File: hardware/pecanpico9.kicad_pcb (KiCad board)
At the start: 4 copper layers, 29.8 x 33.7 mm, 111 parts, among them IC1 SPV1040T, IC2 TPS62260DRVR, IC3 ADP322ACPZ-115-R7, IC4 Si4063-B1B-FM, IC5 STM32F413xG, IC6 EVA-7M, IC7 PAC1720-1-AIA-TR, IC8 LDLN015PU33R, IC9 BME280, P1 CONN_01X25, P2 CONN_01X10, P3 ZX62-B-5PA(33), P4 IPX 2mm, P5 CONN_01X02, P6 IPX 2mm, Q1 FDN306P, X1 KT2016K26000BCW18ZAS

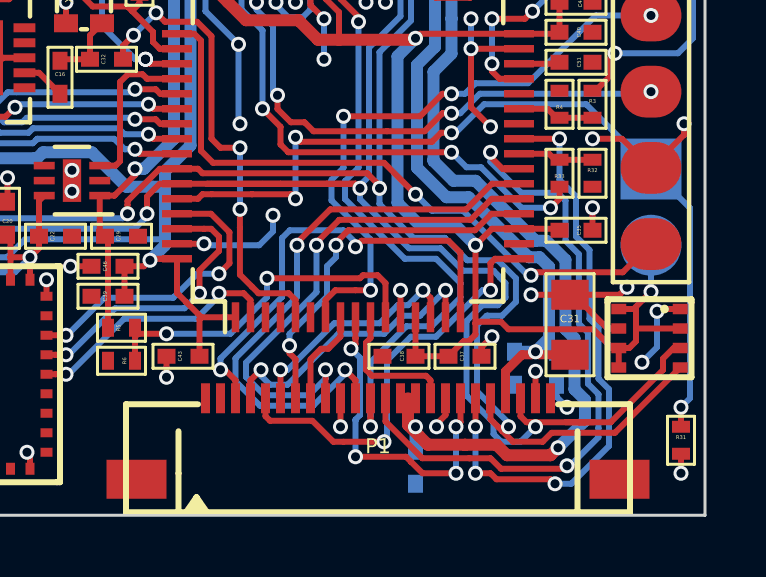
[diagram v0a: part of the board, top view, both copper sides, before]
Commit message: Wiggled parts around
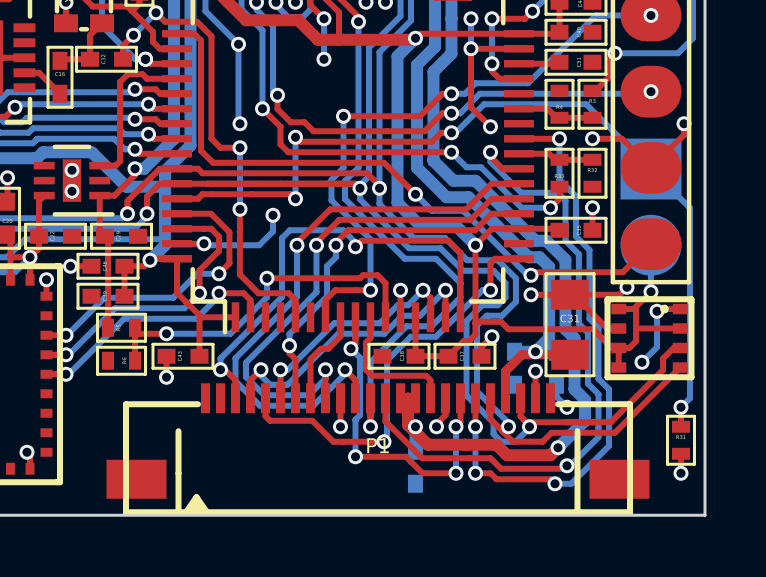
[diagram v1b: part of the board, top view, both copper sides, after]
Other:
- net class Default: clearance 0.15 -> 0.149
- rule trace_clearance: 0.15 -> 0.149
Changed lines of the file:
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@@
     (thickness 1)
     (drawings 30)
-    (tracks 1487)
+    (tracks 1489)
     (zones 0)
     (modules 111)
@@
   (setup
     (last_trace_width 0.2)
-    (trace_clearance 0.15)
+    (trace_clearance 0.149)
     (zone_clearance 0.15)
     (zone_45_only no)
@@
   (net 78 /CAM_PCLK)
   (net_class Default "This is the default net class."
-    (clearance 0.15)
+    (clearance 0.149)
     (trace_width 0.2)
     (via_dia 0.5)
@@
   (via (at 58.35 110.9) (size 0.5) (drill 0.3) (layers F.Cu B.Cu) (net 22))
   (via (at 53.9 111) (size 0.5) (drill 0.3) (layers F.Cu B.Cu) (net 22))
+  (segment (start 71.05 121.65) (end 71.05 121.690002) (width 0.2) (layer B.Cu) (net 23))
+  (segment (start 70.110479 122.149001) (end 69.850999 121.889521) (width 0.2) (layer B.Cu) (net 23))
+  (segment (start 70.249001 117.339521) (end 70.249001 116.860479) (width 0.2) (layer B.Cu) (net 23))
+  (segment (start 71.05 121.690002) (end 70.591001 122.149001) (width 0.2) (layer B.Cu) (net 23))
+  (segment (start 70.591001 122.149001) (end 70.110479 122.149001) (width 0.2) (layer B.Cu) (net 23))
+  (segment (start 69.850999 121.889521) (end 69.850999 121.512477) (width 0.2) (layer B.Cu) (net 23))
+  (segment (start 69.850999 121.512477) (end 68.95199 120.613468) (width 0.2) (layer B.Cu) (net 23))
+  (segment (start 70.249001 116.860479) (end 70.051374 116.662852) (width 0.2) (layer B.Cu) (net 23))
+  (segment (start 68.95199 118.12368) (end 69.476669 117.599001) (width 0.2) (layer B.Cu) (net 23))
+  (segment (start 68.95199 120.613468) (end 68.95199 118.12368) (width 0.2) (layer B.Cu) (net 23))
+  (segment (start 69.476669 117.599001) (end 69.989521 117.599001) (width 0.2) (layer B.Cu) (net 23))
+  (segment (start 69.849384 116.44801) (end 68.830106 116.44801) (width 0.2) (layer B.Cu) (net 23))
+  (segment (start 69.989521 117.599001) (end 70.249001 117.339521) (width 0.2) (layer B.Cu) (net 23))
+  (segment (start 70.051374 116.662852) (end 70.051374 116.65) (width 0.2) (layer B.Cu) (net 23))
+  (segment (start 70.051374 116.65) (end 69.849384 116.44801) (width 0.2) (layer B.Cu) (net 23))
+  (segment (start 68.830106 116.44801) (end 68.083095 115.700999) (width 0.2) (layer B.Cu) (net 23))
+  (segment (start 68.083095 115.700999) (end 67.035907 115.700999) (width 0.2) (layer B.Cu) (net 23))
+  (segment (start 67.035907 115.700999) (end 65.4 114.065092) (width 0.2) (layer B.Cu) (net 23))
+  (segment (start 65.4 114.065092) (end 65.4 113.7) (width 0.2) (layer B.Cu) (net 23))
+  (segment (start 70.951798 121.5) (end 70.851798 121.4) (width 0.2) (layer F.Cu) (net 23))
+  (segment (start 70.851798 121.4) (end 70.75 121.298202) (width 0.2) (layer F.Cu) (net 23))
+  (segment (start 71.05 121.65) (end 71.05 121.598202) (width 0.2) (layer F.Cu) (net 23))
+  (segment (start 71.05 121.598202) (end 70.851798 121.4) (width 0.2) (layer F.Cu) (net 23))
   (segment (start 65.4 113.7) (end 65.4 113.6) (width 0.2) (layer B.Cu) (net 23))
   (segment (start 65.7 109.017838) (end 65.94999 108.767848) (width 0.2) (layer B.Cu) (net 23))
@@
   (segment (start 60.3 113.55) (end 64.3 113.55) (width 0.2) (layer F.Cu) (net 23))
   (segment (start 64.3 113.55) (end 64.30099 113.54901) (width 0.2) (layer F.Cu) (net 23))
-  (segment (start 70.051374 116.662852) (end 70.249001 116.860479) (width 0.2) (layer B.Cu) (net 23))
-  (segment (start 65.4 113.7) (end 65.4 114.065092) (width 0.2) (layer B.Cu) (net 23))
-  (segment (start 69.989521 117.599001) (end 69.476669 117.599001) (width 0.2) (layer B.Cu) (net 23))
-  (segment (start 67.035907 115.700999) (end 68.083095 115.700999) (width 0.2) (layer B.Cu) (net 23))
-  (segment (start 69.849384 116.44801) (end 70.051374 116.65) (width 0.2) (layer B.Cu) (net 23))
-  (segment (start 65.4 114.065092) (end 67.035907 115.700999) (width 0.2) (layer B.Cu) (net 23))
-  (segment (start 68.083095 115.700999) (end 68.830106 116.44801) (width 0.2) (layer B.Cu) (net 23))
-  (segment (start 70.051374 116.65) (end 70.051374 116.662852) (width 0.2) (layer B.Cu) (net 23))
-  (segment (start 68.830106 116.44801) (end 69.849384 116.44801) (width 0.2) (layer B.Cu) (net 23))
-  (segment (start 69.476669 117.599001) (end 68.95199 118.12368) (width 0.2) (layer B.Cu) (net 23))
-  (segment (start 70.249001 116.860479) (end 70.249001 117.339521) (width 0.2) (layer B.Cu) (net 23))
-  (segment (start 70.249001 117.339521) (end 69.989521 117.599001) (width 0.2) (layer B.Cu) (net 23))
-  (segment (start 70.750999 122.149001) (end 71.25 121.65) (width 0.2) (layer B.Cu) (net 23))
-  (segment (start 68.95199 118.12368) (end 68.95199 120.613468) (width 0.2) (layer B.Cu) (net 23))
-  (segment (start 68.95199 120.613468) (end 69.850999 121.512477) (width 0.2) (layer B.Cu) (net 23))
-  (segment (start 69.850999 121.512477) (end 69.850999 121.889521) (width 0.2) (layer B.Cu) (net 23))
-  (segment (start 69.850999 121.889521) (end 70.110479 122.149001) (width 0.2) (layer B.Cu) (net 23))
-  (segment (start 70.110479 122.149001) (end 70.750999 122.149001) (width 0.2) (layer B.Cu) (net 23))
   (segment (start 58.3 114.55) (end 58.3 114.638522) (width 0.2) (layer B.Cu) (net 23))
   (segment (start 58.3 114.638522) (end 57.888511 115.050011) (width 0.2) (layer B.Cu) (net 23))
@@
   (segment (start 72.9 121.5) (end 71.1 121.5) (width 0.2) (layer F.Cu) (net 23))
   (segment (start 71.1 121.5) (end 70.951798 121.5) (width 0.2) (layer F.Cu) (net 23))
-  (segment (start 71.25 121.65) (end 71.1 121.5) (width 0.2) (layer F.Cu) (net 23))
   (segment (start 72.9 121.5) (end 73.2 121.5) (width 0.2) (layer F.Cu) (net 23))
-  (segment (start 70.951798 121.5) (end 70.75 121.298202) (width 0.2) (layer F.Cu) (net 23))
   (segment (start 70.75 120.7) (end 70.75 121.298202) (width 0.2) (layer F.Cu) (net 23))
-  (segment (start 71.101798 121.65) (end 71.25 121.65) (width 0.2) (layer F.Cu) (net 23))
-  (via (at 71.25 121.65) (size 0.5) (drill 0.3) (layers F.Cu B.Cu) (net 23))
+  (via (at 71.05 121.65) (size 0.5) (drill 0.3) (layers F.Cu B.Cu) (net 23))
   (segment (start 58.3 114.25) (end 58.3 114.55) (width 0.2) (layer F.Cu) (net 23))
   (segment (start 65.499001 113.799001) (end 65.4 113.7) (width 0.2) (layer B.Cu) (net 23))
